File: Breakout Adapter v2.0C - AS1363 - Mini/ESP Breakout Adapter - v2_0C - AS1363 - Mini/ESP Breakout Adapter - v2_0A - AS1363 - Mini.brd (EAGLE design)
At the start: 24.3 x 30.6 mm, 27 parts

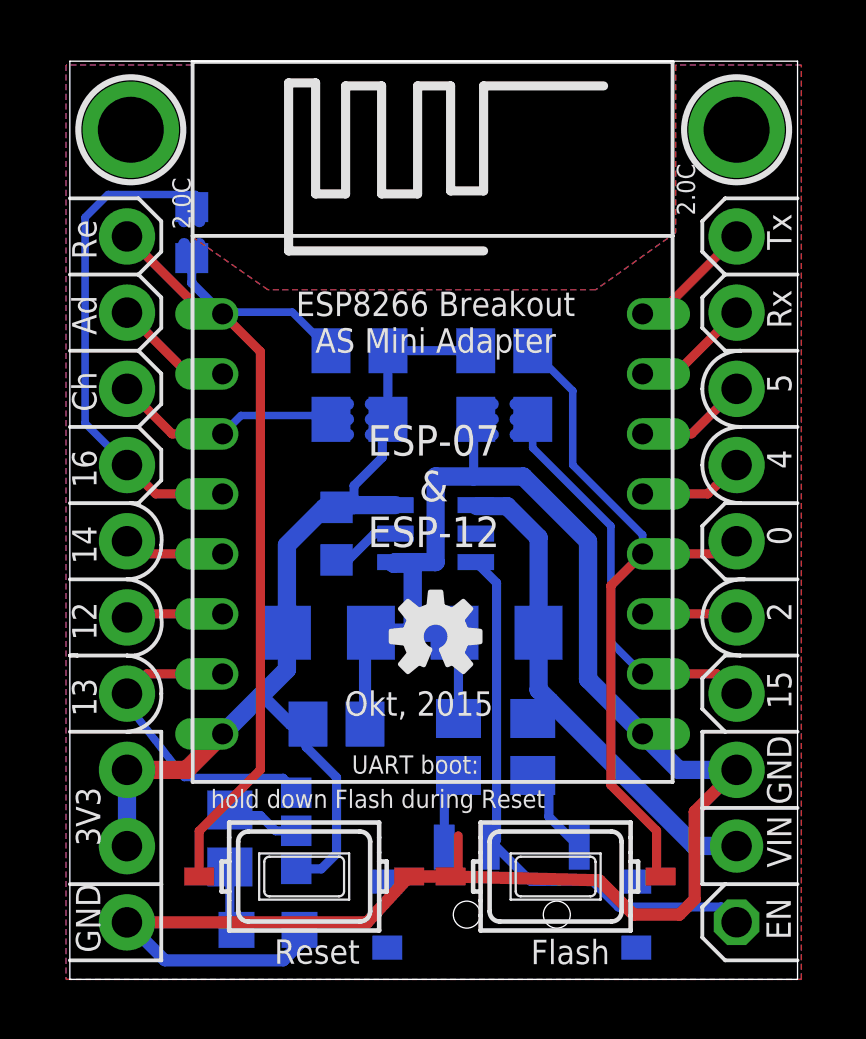
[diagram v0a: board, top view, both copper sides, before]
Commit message: mini änderung
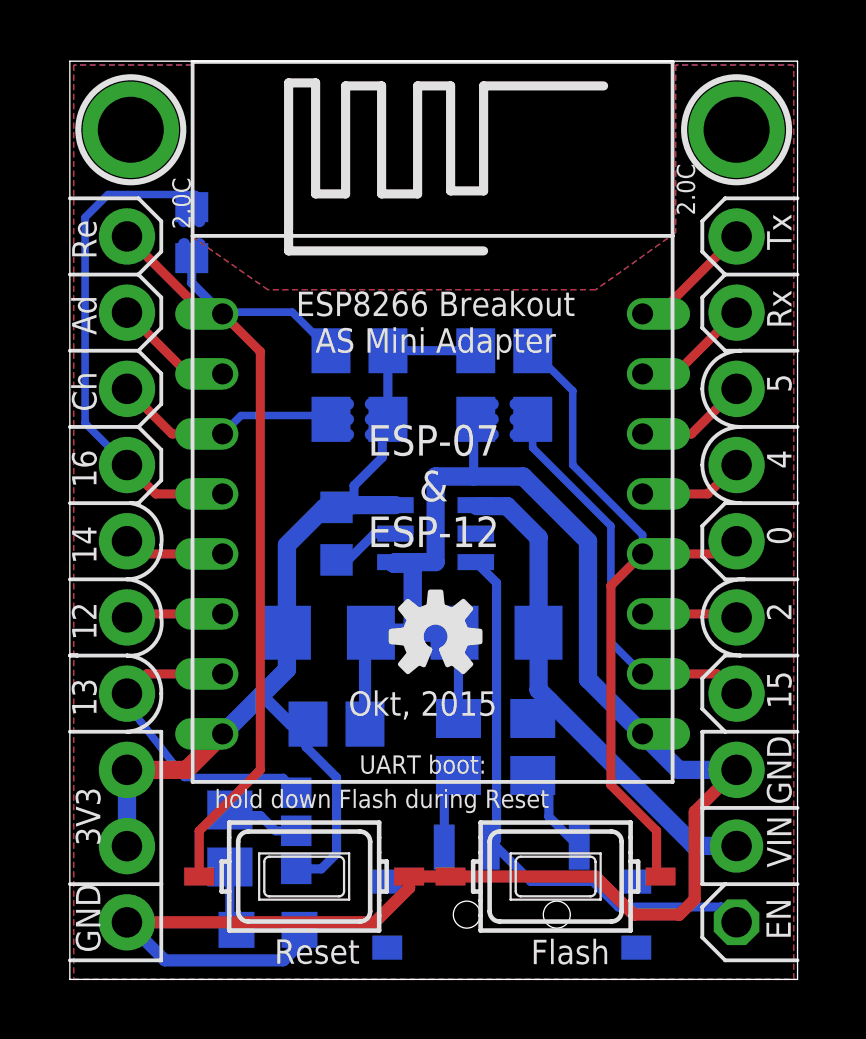
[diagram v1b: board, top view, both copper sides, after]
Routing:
- net GND: track 70.3 -> 69.0 mm
- net RESET: track 32.5 -> 32.0 mm
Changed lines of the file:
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@@
 <text x="23.495" y="25.654" size="0.8128" layer="21" ratio="12" rot="R270">Tx</text>
 <text x="4.2799" y="25.1333" size="0.6096" layer="21" ratio="12" rot="R90">2.0C</text>
-<text x="9.41340625" y="8.916303125" size="0.8128" layer="21">Okt, 2015</text>
+<text x="9.54040625" y="8.916303125" size="0.8128" layer="21">Okt, 2015</text>
 <text x="23.47268125" y="2.835553125" size="0.8128" layer="21" ratio="12" rot="R270">EN</text>
 <wire x1="24.511" y1="8.382" x2="22.098" y2="8.382" width="0.127" layer="21"/>
@@
 <text x="12.446" y="23.0505" size="0.8128" layer="21" ratio="12" align="top-center">ESP8266 Breakout
 AS Mini Adapter</text>
-<text x="4.953" y="5.842" size="0.6096" layer="21" ratio="12">hold down Flash during Reset</text>
-<text x="9.652" y="6.985" size="0.6096" layer="21" ratio="12">UART boot:</text>
+<text x="5.08" y="5.842" size="0.6096" layer="21" ratio="12">hold down Flash during Reset</text>
+<text x="9.906" y="6.985" size="0.6096" layer="21" ratio="12">UART boot:</text>
 </plain>
 <attributes>
@@
 <wire x1="0.762" y1="25.527" x2="0.762" y2="18.669" width="0.254" layer="16"/>
 <wire x1="0.762" y1="18.669" x2="2.159" y2="17.272" width="0.254" layer="16"/>
-<wire x1="4.445" y1="26.289" x2="4.445" y2="26.223" width="0.254" layer="16"/>
-<wire x1="4.445" y1="26.223" x2="4.318" y2="25.869" width="0.254" layer="16"/>
 <wire x1="4.064" y1="25.4" x2="4.064" y2="25.908" width="0.4064" layer="16"/>
 <wire x1="4.572" y1="25.4" x2="4.572" y2="26.162" width="0.4064" layer="16"/>
 <wire x1="4.064" y1="25.908" x2="4.511" y2="25.908" width="0.3048" layer="16"/>
-<wire x1="4.511" y1="25.908" x2="4.318" y2="25.869" width="0.3048" layer="16"/>
-<wire x1="4.572" y1="26.162" x2="4.318" y2="25.869" width="0.3048" layer="16"/>
+<wire x1="4.445" y1="26.289" x2="4.445" y2="25.996" width="0.254" layer="16"/>
+<wire x1="4.445" y1="25.996" x2="4.318" y2="25.869" width="0.254" layer="16"/>
+<wire x1="4.572" y1="26.162" x2="4.572" y2="26.123" width="0.254" layer="16"/>
+<wire x1="4.572" y1="26.123" x2="4.318" y2="25.869" width="0.254" layer="16"/>
+<wire x1="4.511" y1="25.908" x2="4.357" y2="25.908" width="0.254" layer="16"/>
+<wire x1="4.357" y1="25.908" x2="4.318" y2="25.869" width="0.254" layer="16"/>
 </signal>
 <signal name="GPIO14">
@@
 <wire x1="13.782" y1="18.796" x2="13.716" y2="18.73" width="0.254" layer="16"/>
 <wire x1="13.716" y1="18.73" x2="13.716" y2="16.891" width="0.3048" layer="16"/>
-<wire x1="2.157159375" y1="2.028784375" x2="10.164284375" y2="2.028784375" width="0.4064" layer="1"/>
-<wire x1="10.164284375" y1="2.028784375" x2="11.5645" y2="3.556" width="0.4064" layer="1"/>
+<wire x1="2.157159375" y1="2.028784375" x2="10.418284375" y2="2.028784375" width="0.4064" layer="1"/>
 <wire x1="11.5645" y1="3.556" x2="12.9465" y2="3.556" width="0.4064" layer="1"/>
 <wire x1="19.346" y1="8.31" x2="20.543359375" y2="7.112640625" width="0.6096" layer="16"/>
@@
 <wire x1="14.224" y1="18.796" x2="14.224" y2="18.288" width="0.3048" layer="16"/>
 <wire x1="13.782" y1="18.796" x2="14.224" y2="18.796" width="0.3048" layer="16"/>
-<wire x1="12.9465" y1="3.556" x2="17.907" y2="3.429" width="0.4064" layer="1"/>
-<wire x1="17.907" y1="3.429" x2="19.05" y2="2.286" width="0.4064" layer="1"/>
+<wire x1="17.78" y1="3.556" x2="19.05" y2="2.286" width="0.4064" layer="1"/>
 <wire x1="19.05" y1="2.286" x2="20.574" y2="2.286" width="0.4064" layer="1"/>
 <wire x1="20.574" y1="2.286" x2="21.082" y2="2.794" width="0.4064" layer="1"/>
@@
 <wire x1="7.366" y1="0.762" x2="3.42394375" y2="0.762" width="0.4064" layer="16"/>
 <wire x1="3.42394375" y1="0.762" x2="2.157159375" y2="2.028784375" width="0.4064" layer="16"/>
-<polygon width="0.3048" layer="16">
-<vertex x="0.127" y="0.127"/>
-<vertex x="24.638" y="0.127"/>
-<vertex x="24.638" y="30.607"/>
+<polygon width="0.3048" layer="1">
+<vertex x="0.381" y="0.127"/>
+<vertex x="24.384" y="0.127"/>
+<vertex x="24.384" y="30.607"/>
 <vertex x="20.447" y="30.607"/>
 <vertex x="20.447" y="25.019"/>
@@
 <vertex x="4.318" y="24.892"/>
 <vertex x="4.318" y="30.607"/>
-<vertex x="0.127" y="30.607"/>
+<vertex x="0.381" y="30.607"/>
 </polygon>
-<wire x1="13.2005" y1="3.6415" x2="13.2005" y2="4.9115" width="0.3048" layer="1"/>
-<wire x1="13.2005" y1="3.6415" x2="13.159" y2="3.6415" width="0.3048" layer="1"/>
-<wire x1="13.159" y1="3.6415" x2="12.9465" y2="3.556" width="0.3048" layer="1"/>
-<polygon width="0.3048" layer="1">
-<vertex x="0.127" y="0.127"/>
-<vertex x="24.638" y="0.127"/>
-<vertex x="24.638" y="30.607"/>
+<wire x1="12.9465" y1="3.556" x2="17.78" y2="3.556" width="0.4064" layer="1"/>
+<wire x1="11.5645" y1="3.556" x2="11.5645" y2="3.175" width="0.4064" layer="1"/>
+<wire x1="11.5645" y1="3.175" x2="10.418284375" y2="2.028784375" width="0.4064" layer="1"/>
+<polygon width="0.3048" layer="16">
+<vertex x="0.381" y="0.127"/>
+<vertex x="24.384" y="0.127"/>
+<vertex x="24.384" y="30.607"/>
 <vertex x="20.447" y="30.607"/>
 <vertex x="20.447" y="25.019"/>
@@
 <vertex x="4.318" y="24.892"/>
 <vertex x="4.318" y="30.607"/>
-<vertex x="0.127" y="30.607"/>
+<vertex x="0.381" y="30.607"/>
 </polygon>
 </signal>
@@
 <wire x1="4.5645" y1="5.0725" x2="6.604" y2="7.112" width="0.3048" layer="1"/>
 <wire x1="4.064" y1="24.638" x2="4.064" y2="24.384" width="0.4064" layer="16"/>
-<wire x1="4.572" y1="24.638" x2="4.318" y2="24.169" width="0.4064" layer="16"/>
-<wire x1="4.318" y1="24.169" x2="4.572" y2="24.384" width="0.4064" layer="16"/>
-<wire x1="4.572" y1="24.638" x2="4.064" y2="24.384" width="0.3048" layer="16"/>
+<wire x1="4.572" y1="24.638" x2="4.572" y2="24.423" width="0.4064" layer="16"/>
+<wire x1="4.572" y1="24.423" x2="4.318" y2="24.169" width="0.4064" layer="16"/>
+<wire x1="4.318" y1="24.169" x2="4.279" y2="24.169" width="0.4064" layer="16"/>
+<wire x1="4.279" y1="24.169" x2="4.064" y2="24.384" width="0.4064" layer="16"/>
 </signal>
 <signal name="GPIO13">
